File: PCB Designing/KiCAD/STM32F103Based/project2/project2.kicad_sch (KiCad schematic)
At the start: 38 parts, among them J1 TYPE_C_31_M_12, SW1 NRST, SW2 BOOT, U1 ESP32-C3, U2 W25Q16JVSS, U3 AMS1117-3.3, U4 USBLC6-2SC6, Y1 40MHz

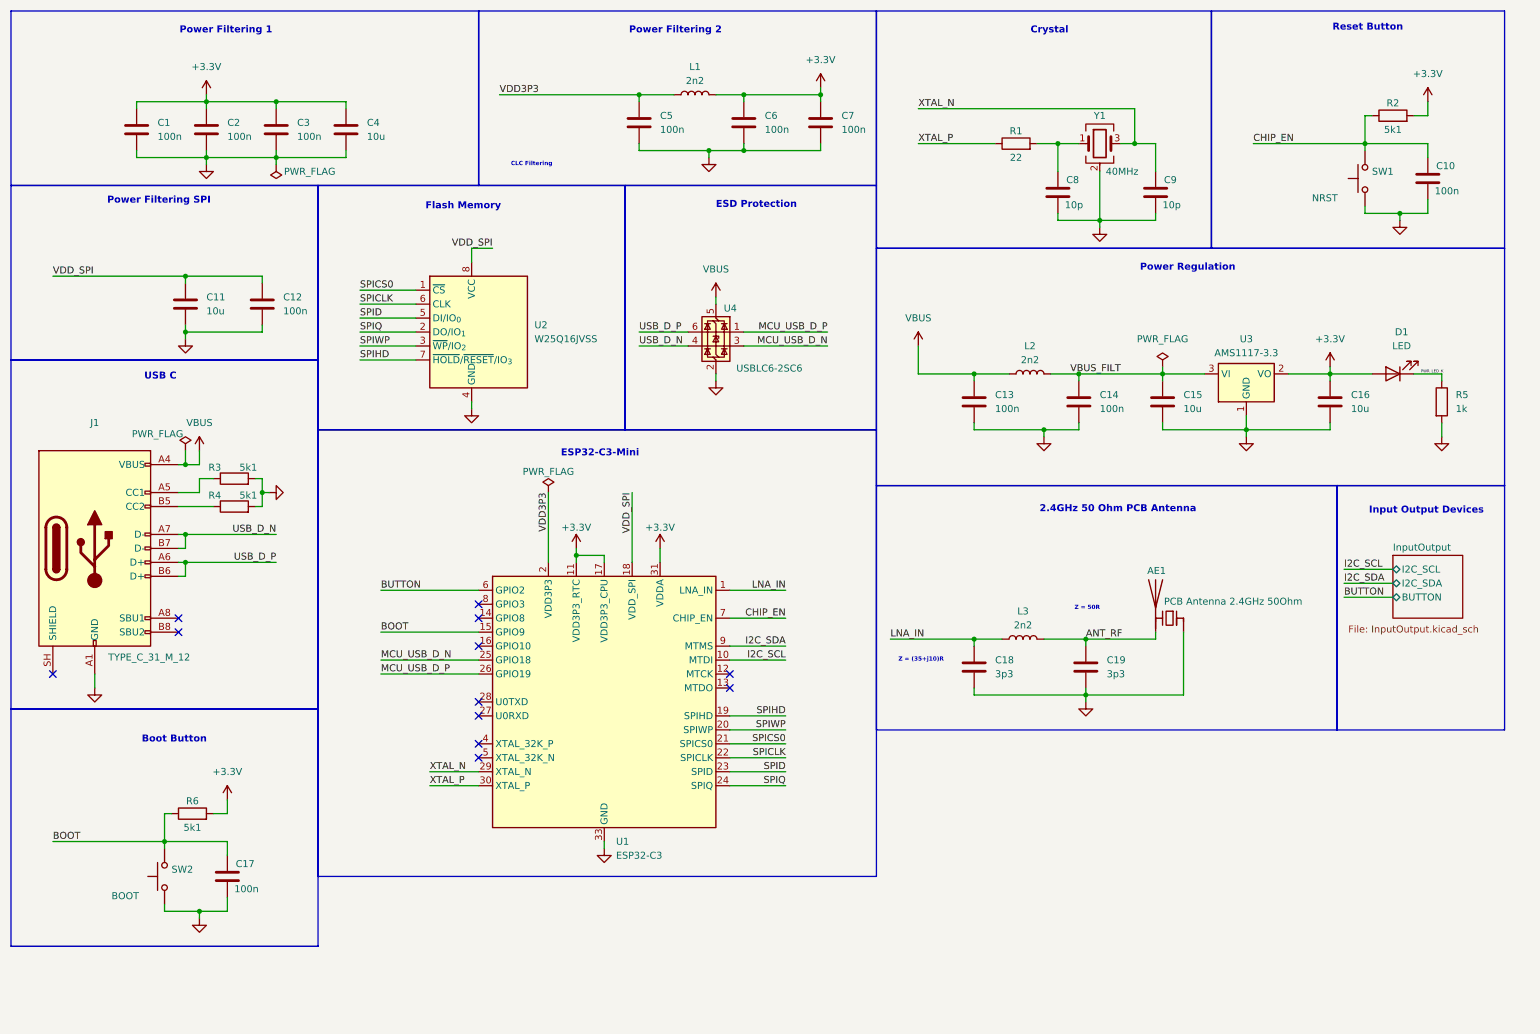
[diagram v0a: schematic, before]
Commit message: Schematics and Footprint Assigned
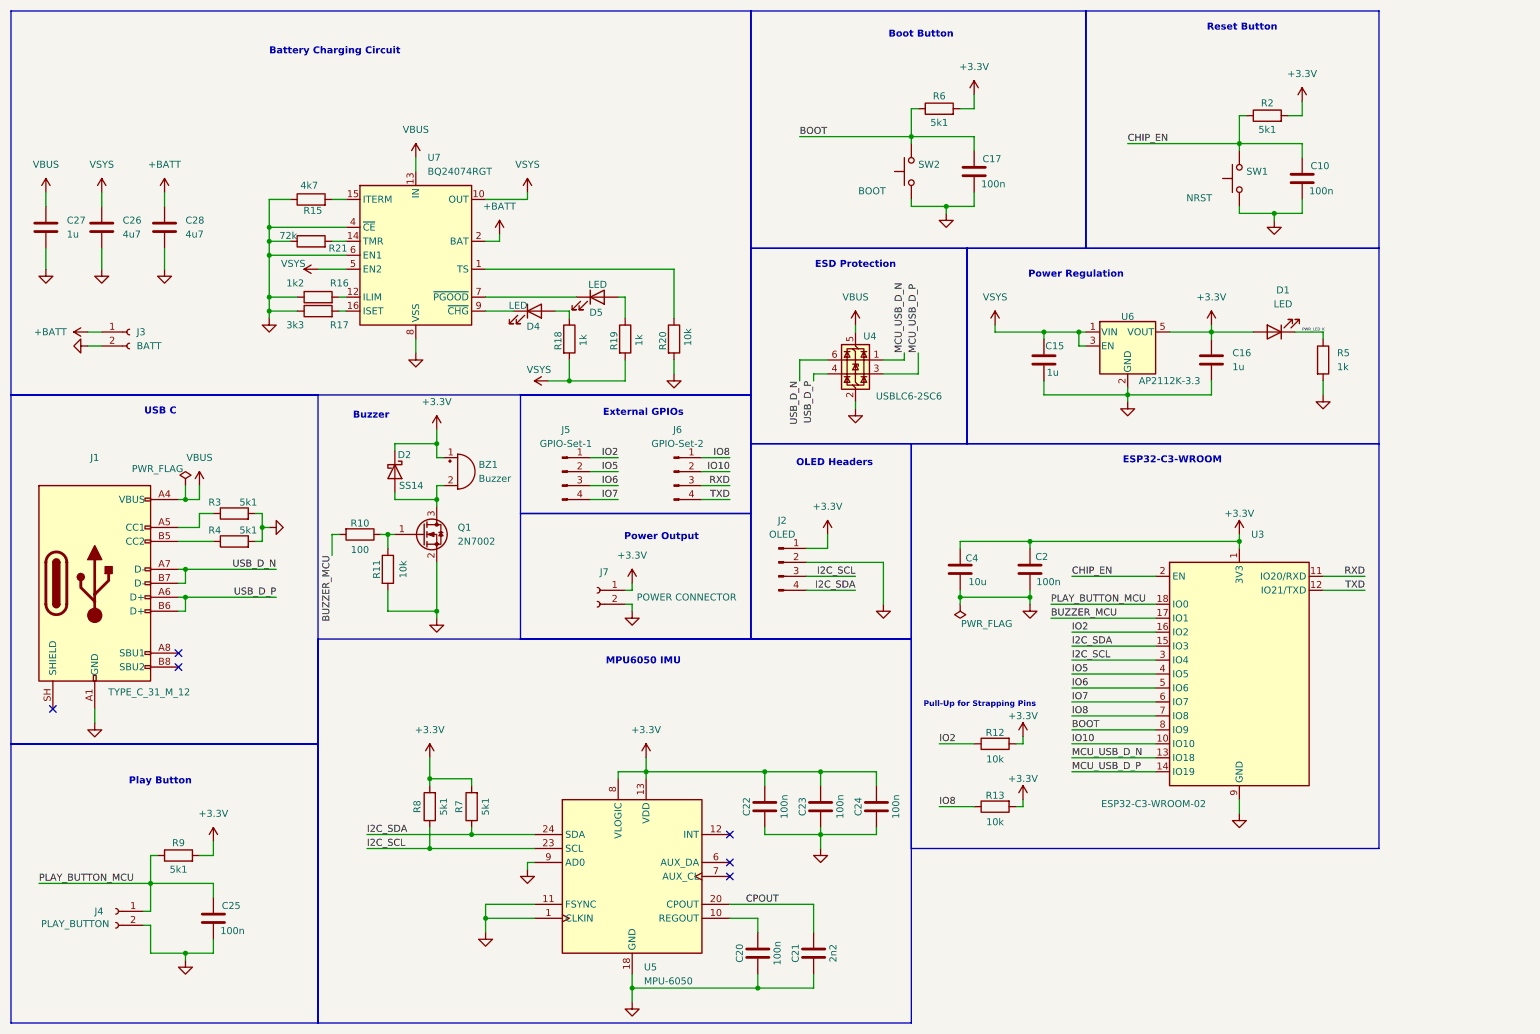
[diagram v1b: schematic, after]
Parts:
- removed AE1: PCB Antenna 2.4GHz 50Ohm, symbol Device:Antenna_Chip
- removed C1, C12, C13, C14, C3, C5, C6, C7: 100n, symbol Device:C
- removed C11: 10u, symbol Device:C
- removed C18, C19: 3p3, symbol Device:C
- removed C8, C9: 10p, symbol Device:C
- removed L1, L2, L3: 2n2, symbol Device:L
- removed R1: 22, symbol Device:R
- removed U1: ESP32-C3, Package_DFN_QFN:QFN-32-1EP_5x5mm_P0.5mm_EP3.7x3.7mm, symbol MCU_Espressif:ESP32-C3
- removed U2: W25Q16JVSS, Package_SO:SOIC-8_5.3x5.3mm_P1.27mm, symbol Memory_Flash:W25Q16JVSS
- removed U3: AMS1117-3.3, Package_TO_SOT_SMD:SOT-223-3_TabPin2, symbol Regulator_Linear:AMS1117-3.3
- removed Y1: 40MHz, symbol Device:Crystal_GND24
- added BZ1: Buzzer, Buzzer_Beeper:Buzzer_CUI_CPT-9019S-SMT, symbol Device:Buzzer
- added C20, C22, C23, C24, C25: 100n, Capacitor_SMD:C_0603_1608Metric, symbol Device:C
- added C21: 2n2, Capacitor_SMD:C_0603_1608Metric, symbol Device:C
- added C26, C28: 4u7, Capacitor_SMD:C_0603_1608Metric, symbol Device:C
- added C27: 1u, Capacitor_SMD:C_0603_1608Metric, symbol Device:C
- added D2: SS14, Diode_SMD:D_SMA, symbol Diode:SS14
- added D4, D5: LED, LED_SMD:LED_0805_2012Metric, symbol Device:LED
- added J2: OLED, Connector_PinHeader_2.54mm:PinHeader_1x04_P2.54mm_Vertical, symbol Connector:Conn_01x04_Pin
- added J3: BATT, Connector_JST:JST_PH_B2B-PH-K_1x02_P2.00mm_Vertical, symbol Connector:Conn_01x02_Socket
- added J4: PLAY_BUTTON, Connector_PinHeader_2.54mm:PinHeader_1x02_P2.54mm_Vertical, symbol Connector:Conn_01x02_Socket
- added J5: GPIO-Set-1, Connector_PinHeader_2.54mm:PinHeader_1x04_P2.54mm_Vertical, symbol Connector:Conn_01x04_Pin
- added J6: GPIO-Set-2, Connector_PinHeader_2.54mm:PinHeader_1x04_P2.54mm_Vertical, symbol Connector:Conn_01x04_Pin
- added J7: POWER CONNECTOR, Connector_PinHeader_2.54mm:PinHeader_1x02_P2.54mm_Vertical, symbol Connector:Conn_01x02_Socket
- added Q1: 2N7002, Package_TO_SOT_SMD:SOT-23, symbol Transistor_FET:2N7002
- added R10: 100, Resistor_SMD:R_0603_1608Metric, symbol Device:R
- added R11, R12, R13, R20: 10k, Resistor_SMD:R_0603_1608Metric, symbol Device:R
- added R15: 4k7, Resistor_SMD:R_0603_1608Metric, symbol Device:R
- added R16: 1k2, Resistor_SMD:R_0603_1608Metric, symbol Device:R
- added R17: 3k3, Resistor_SMD:R_0603_1608Metric, symbol Device:R
- added R18, R19: 1k, Resistor_SMD:R_0603_1608Metric, symbol Device:R
- added R21: 72k, Resistor_SMD:R_0603_1608Metric, symbol Device:R
- added R7, R8, R9: 5k1, Resistor_SMD:R_0603_1608Metric, symbol Device:R
- added U3: ESP32-C3-WROOM-02, RF_Module:ESP32-C3-WROOM-02, symbol RF_Module:ESP32-C3-WROOM-02
- added U5: MPU-6050, Sensor_Motion:InvenSense_QFN-24_4x4mm_P0.5mm, symbol Sensor_Motion:MPU-6050
- added U6: AP2112K-3.3, Package_TO_SOT_SMD:SOT-23-5, symbol Regulator_Linear:AP2112K-3.3
- added U7: BQ24074RGT, Package_DFN_QFN:VQFN-16-1EP_3x3mm_P0.5mm_EP1.6x1.6mm, symbol Battery_Management:BQ24074RGT
- C10, C17, C2, C4: footprint (none) -> Capacitor_SMD:C_0603_1608Metric
- C15, C16: value 10u -> 1u; footprint (none) -> Capacitor_SMD:C_0603_1608Metric
- D1: footprint (none) -> LED_SMD:LED_0805_2012Metric
- J1: footprint (none) -> Connector_USB:USB_C_Receptacle_HRO_TYPE-C-31-M-12
- R2, R3, R4, R5, R6: footprint (none) -> Resistor_SMD:R_0603_1608Metric
- SW1, SW2: footprint (none) -> Button_Switch_SMD:SW_SPST_PTS645Sx43SMTR92
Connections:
- net +3.3V: now also BZ1.1 (+), C22.2, C23.2, C24.2, D2.1 (K), J2.1 (Pin_1), J7.1 (Pin_1), R12.2, R13.2, R7.2, R8.2, R9.2, U3.1 (3V3), U5.13 (VDD), U5.8 (VLOGIC), U6.5 (VOUT)
- net BOOT: now also U3.8 (IO9)
- net CHIP_EN: now also U3.2 (EN)
- net GND: now also C20.1, C21.1, C22.1, C23.1, C24.1, C25.2, C26.2, C27.2, C28.2, J2.2 (Pin_2), J3.2 (Pin_2), J4.2 (Pin_2), J7.2 (Pin_2), Q1.2 (S), R11.2, R15.1, R16.1, R17.1, R20.2, R21.1, U3.19 (GND), U3.9 (GND), U5.1 (CLKIN), U5.11 (FSYNC), U5.18 (GND), U5.9 (AD0), U6.2 (GND), U7.17 (VSS), U7.4 (~{CE}), U7.6 (EN1), U7.8 (VSS)
- net I2C_SCL: now also J2.3 (Pin_3), R8.1, U3.3 (IO4), U5.23 (SCL)
- net I2C_SDA: now also J2.4 (Pin_4), R7.1, U3.15 (IO3), U5.24 (SDA)
- net MCU_USB_D_N: now also U4.1 (I/O1), U3.13 (IO18); no longer U4.3 (I/O2)
- net MCU_USB_D_P: now also U4.3 (I/O2), U3.14 (IO19); no longer U4.1 (I/O1)
- net USB_D_N: now also U4.6 (I/O1); no longer U4.4 (I/O2)
- net USB_D_P: now also U4.4 (I/O2); no longer U4.6 (I/O1)
- net VBUS: now also C27.1, U7.13 (IN)
- net VBUS_FILT renamed VSYS
- net VSYS: now also C26.1, R18.2, R19.2, U6.1 (VIN), U6.3 (EN), U7.10 (OUT), U7.11 (OUT), U7.5 (EN2)
- new net: D4.2 (A), R18.1
- new net: R15.2, U7.15 (ITERM)
- new net: Q1.1 (G), R10.1, R11.1
- new net: BZ1.2 (-), D2.2 (A), Q1.3 (D)
- new net: C20.2, U5.10 (REGOUT)
- new net: R20.1, U7.1 (TS)
- new net: R21.2, U7.14 (TMR)
- new net: D4.1 (K), U7.9 (~{CHG})
- new net: R16.2, U7.12 (ILIM)
- new net: R17.2, U7.16 (ISET)
- new net: D5.1 (K), U7.7 (~{PGOOD})
- new net: D5.2 (A), R19.1
- new net +BATT: C28.1, J3.1 (Pin_1), U7.2 (BAT), U7.3 (BAT)
- new net BUZZER_MCU: R10.2, U3.17 (IO1)
- new net CPOUT: C21.2, U5.20 (CPOUT)
- new net IO10: J6.2 (Pin_2), U3.10 (IO10)
- new net IO2: J5.1 (Pin_1), R12.1, U3.16 (IO2)
- new net IO5: J5.2 (Pin_2), U3.4 (IO5)
- new net IO6: J5.3 (Pin_3), U3.5 (IO6)
- new net IO7: J5.4 (Pin_4), U3.6 (IO7)
- new net IO8: J6.1 (Pin_1), R13.1, U3.7 (IO8)
- new net PLAY_BUTTON_MCU: C25.1, J4.1 (Pin_1), R9.1, U3.18 (IO0)
- new net RXD: J6.3 (Pin_3), U3.11 (IO20/RXD)
- new net TXD: J6.4 (Pin_4), U3.12 (IO21/TXD)
- no-connect marks 12 -> 6
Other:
- removed sheet InputOutput
- note added: "Battery Charging Circuit"
- note added: "Buzzer"
- note added: "ESP32-C3-WROOM"
- note added: "External GPIOs"
- note added: "MPU6050 IMU"
- note added: "OLED Headers"
- note added: "Play Button"
- note added: "Power Output"
- note added: "Pull-Up for Strapping Pins"
- note removed: "2.4GHz 50 Ohm PCB Antenna"
- note removed: "CLC Filtering"
- note removed: "Crystal"
- note removed: "ESP32-C3-Mini"
- note removed: "Flash Memory"
- note removed: "Input Output Devices"
- note removed: "Power Filtering 1"
- note removed: "Power Filtering 2"
- note removed: "Power Filtering SPI"
- note removed: "Z = (35+j10)R"
- note removed: "Z = 50R"
- moved on the sheet: C10, C17, J1, R2, R3, R4, R6, SW1, SW2
